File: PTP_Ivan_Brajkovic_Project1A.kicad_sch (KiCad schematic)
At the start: 25 parts, among them J1 Screw_Terminal_01x02, SW1 SW_Push_Dual_x2, SW2 SW2, U1 LM2574N-5, U1 NE555P

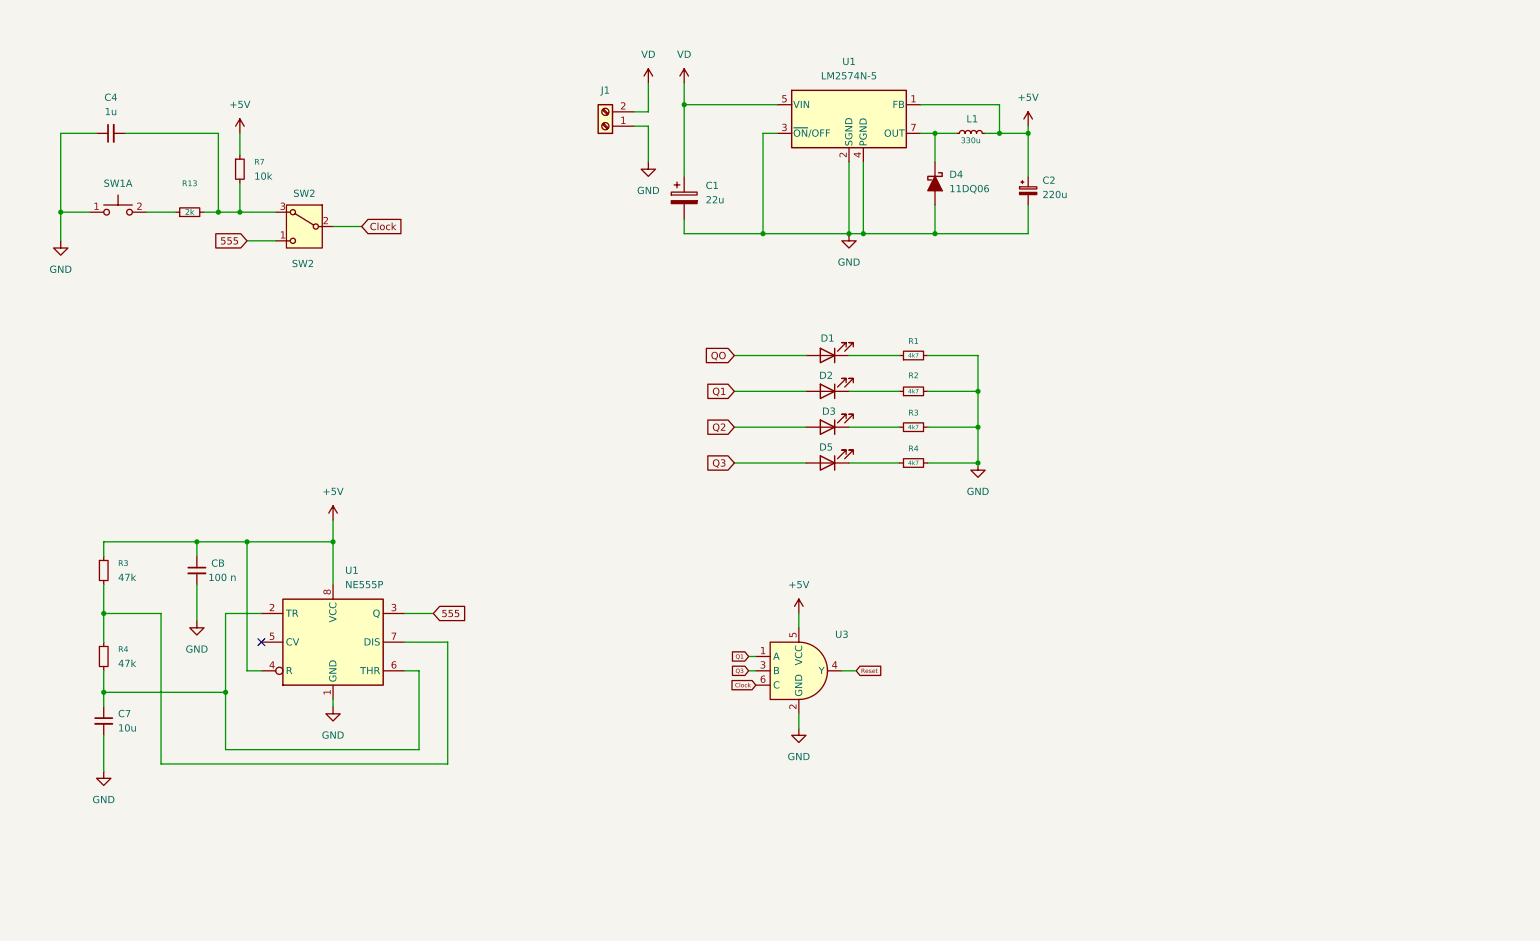
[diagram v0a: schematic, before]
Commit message: LV4 DONE
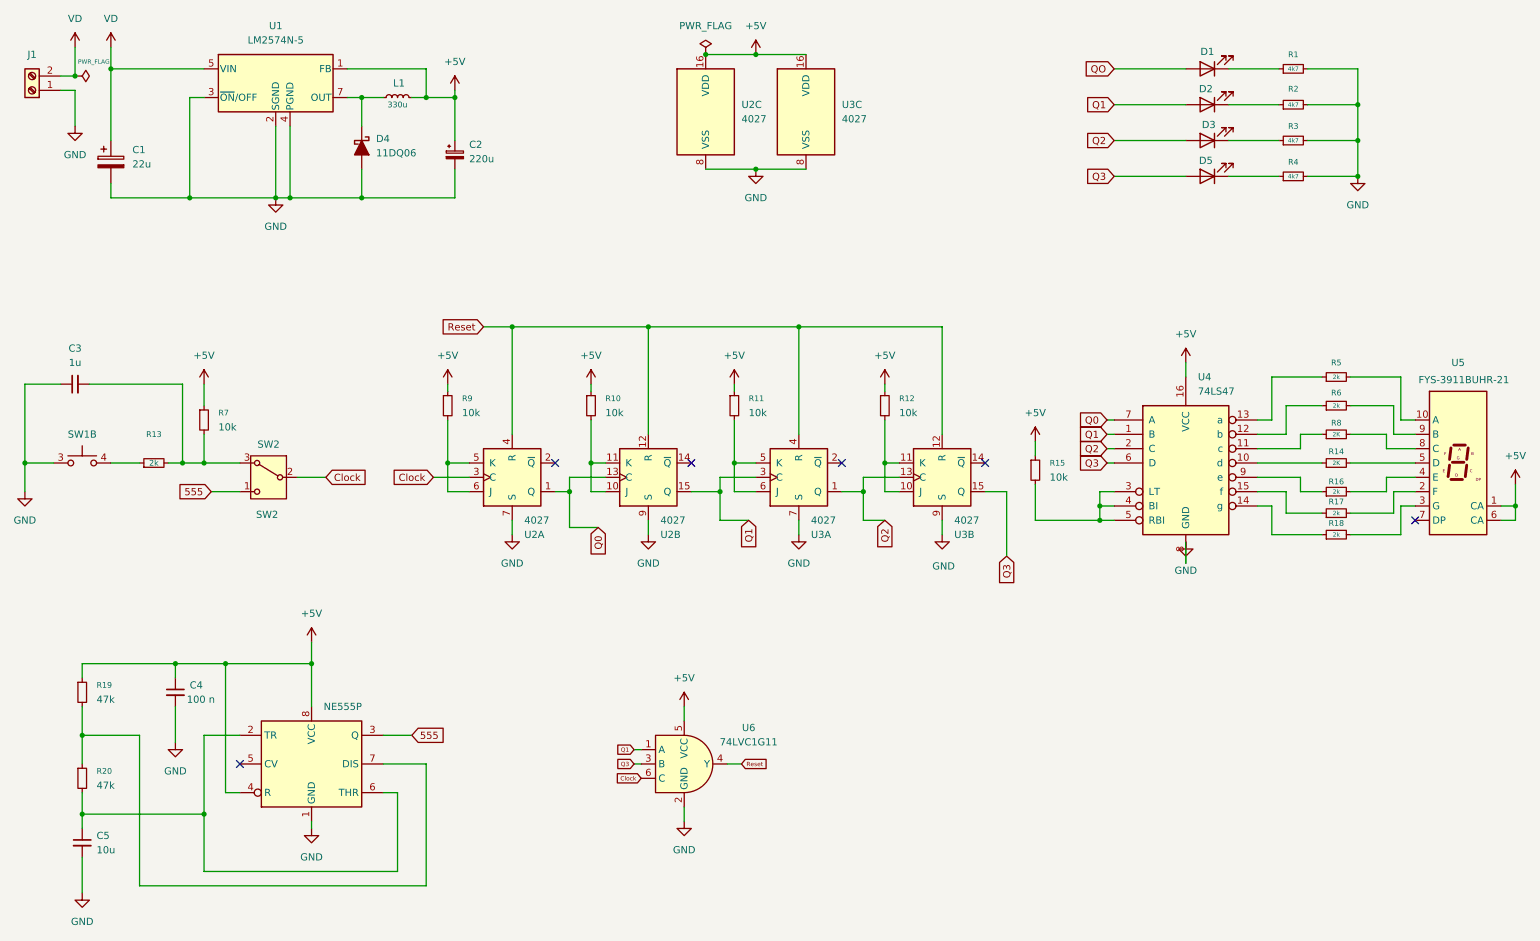
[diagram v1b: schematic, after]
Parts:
- added R10, R11, R12, R15, R9: 10k, symbol Device:R_Small
- added R14, R8: 2K, Resistor_SMD:R_1206_3216Metric_Pad1.30x1.75mm_HandSolder, symbol Device:R_Small
- added R16, R17, R5, R6: 2k, Resistor_SMD:R_1206_3216Metric_Pad1.30x1.75mm_HandSolder, symbol Device:R_Small
- added R18: 2k, symbol Device:R_Small
- added U2, U3: 4027, symbol 4xxx:4027
- added U4: 74LS47, Package_DIP:DIP-16_W7.62mm_Socket_LongPads, symbol 74xx:74LS47
- added U5: FYS-3911BUHR-21, Display_7Segment:HDSP-7401, symbol Display_Character:HDSP-7401
- U6: renamed from U3; value ~ -> 74LVC1G11
- renumbered C4 to C3, CB to C4, C7 to C5, R3 to R19, R4 to R20, U1 to U7
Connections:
- net +5V: now also R10.1, R11.1, R12.1, R15.1, R9.1, U2.16 (VDD), U3.16 (VDD), U4.16 (VCC), U5.1 (CA), U5.6 (CA)
- net Clock: now also U2.3 (C)
- net GND: now also SW1.3 (C), U2.7 (S), U2.8 (VSS), U2.9 (S), U3.7 (S), U3.8 (VSS), U3.9 (S), U4.8 (GND); no longer SW1.1 (C)
- net Q1: now also U2.15 (Q), U3.3 (C), U4.1 (B)
- net Q2: now also U3.1 (Q), U3.13 (C), U4.2 (C)
- net Q3: now also U3.15 (Q), U4.6 (D)
- net Reset: now also U2.12 (R), U2.4 (R), U3.12 (R), U3.4 (R)
- net at R13.1: now also SW1.4 (D); no longer SW1.2 (D)
- new net: R11.2, U3.5 (K), U3.6 (J)
- new net: R14.1, U4.10 (d)
- new net: R14.2, U5.5 (D)
- new net: R12.2, U3.10 (J), U3.11 (K)
- new net: R9.2, U2.5 (K), U2.6 (J)
- new net: R17.1, U4.15 (f)
- new net: R17.2, U5.2 (F)
- new net: R18.1, U4.14 (g)
- new net: R18.2, U5.3 (G)
- new net: R5.2, U5.10 (A)
- new net: R16.2, U5.4 (E)
- new net: R8.2, U5.8 (C)
- new net: R6.2, U5.9 (B)
- new net: R16.1, U4.9 (e)
- new net: R6.1, U4.12 (b)
- new net: R8.1, U4.11 (c)
- new net: R5.1, U4.13 (a)
- new net: R15.2, U4.3 (LT), U4.4 (BI), U4.5 (RBI)
- new net: R10.2, U2.10 (J), U2.11 (K)
- new net Q0: U2.1 (Q), U2.13 (C), U4.7 (A)
- no-connect marks 1 -> 6
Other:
- moved on the sheet: C1, C2, C3, C4, C5, D1, D2, D3, D4, D5, J1, L1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
